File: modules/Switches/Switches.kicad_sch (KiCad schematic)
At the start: 0 parts

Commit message: Switches - module design - wip
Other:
- title: Eurorack [thing] -> Switches
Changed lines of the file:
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@@
   (paper "A4")
   (title_block
-    (title "Eurorack [thing]")
-    (rev "0.1")
+    (title "Switches")
+    (date "2023-10-12")
+    (rev "1.0")
     (company "Len Popp")
     (comment 1 "Copyright © 2023 Len Popp CC BY")
-    (comment 2 "Eurorack [thing] module - 8HP")
+    (comment 2 "Eurorack muting module module - 8HP")
   )
   (text "All fixed resistors are 1% tolerance unless otherwise specified.\nAll eletrolytic capacitors are rated for 25VDC unless otherwise specified."

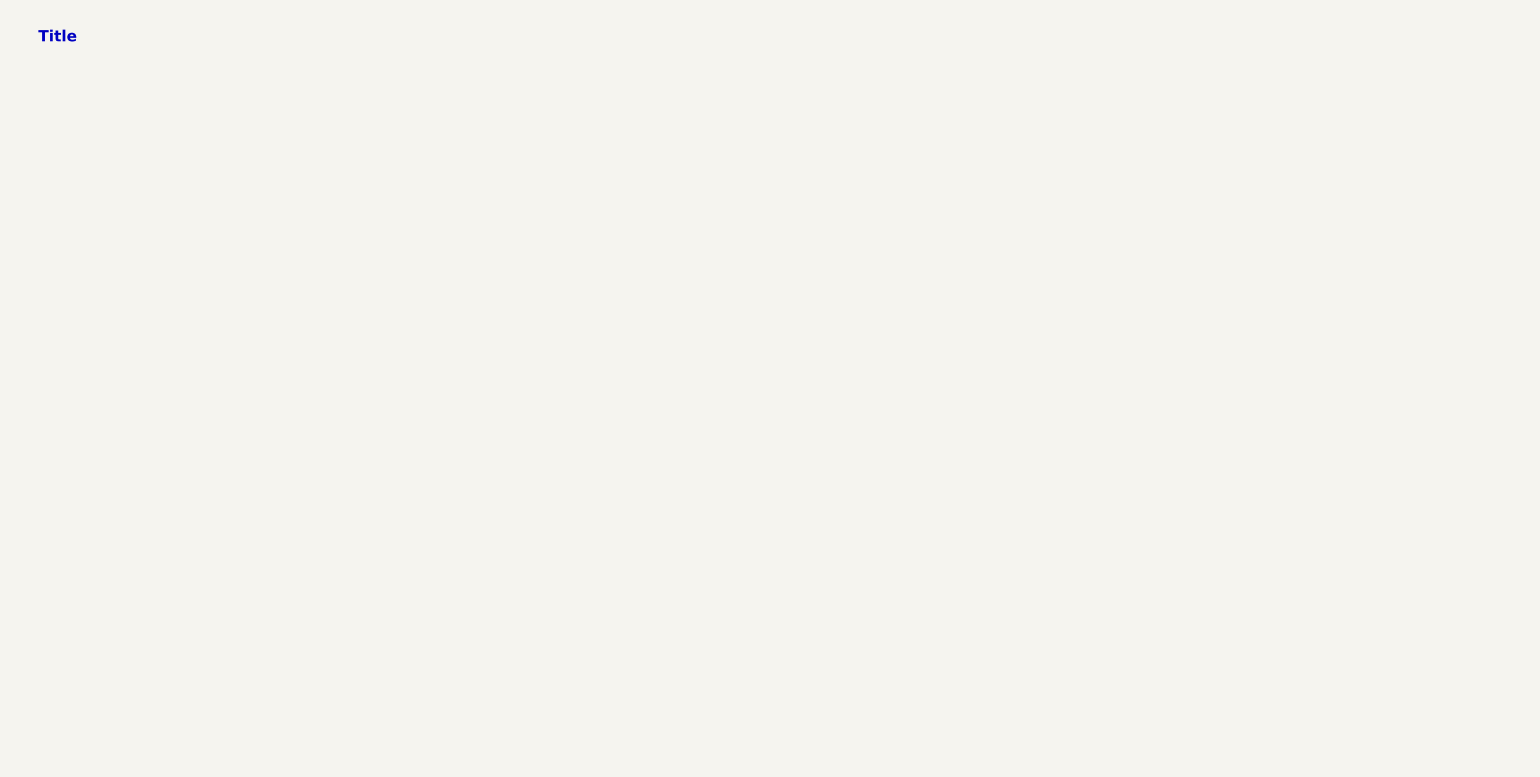
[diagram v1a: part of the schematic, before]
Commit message: Switches - module design - wip
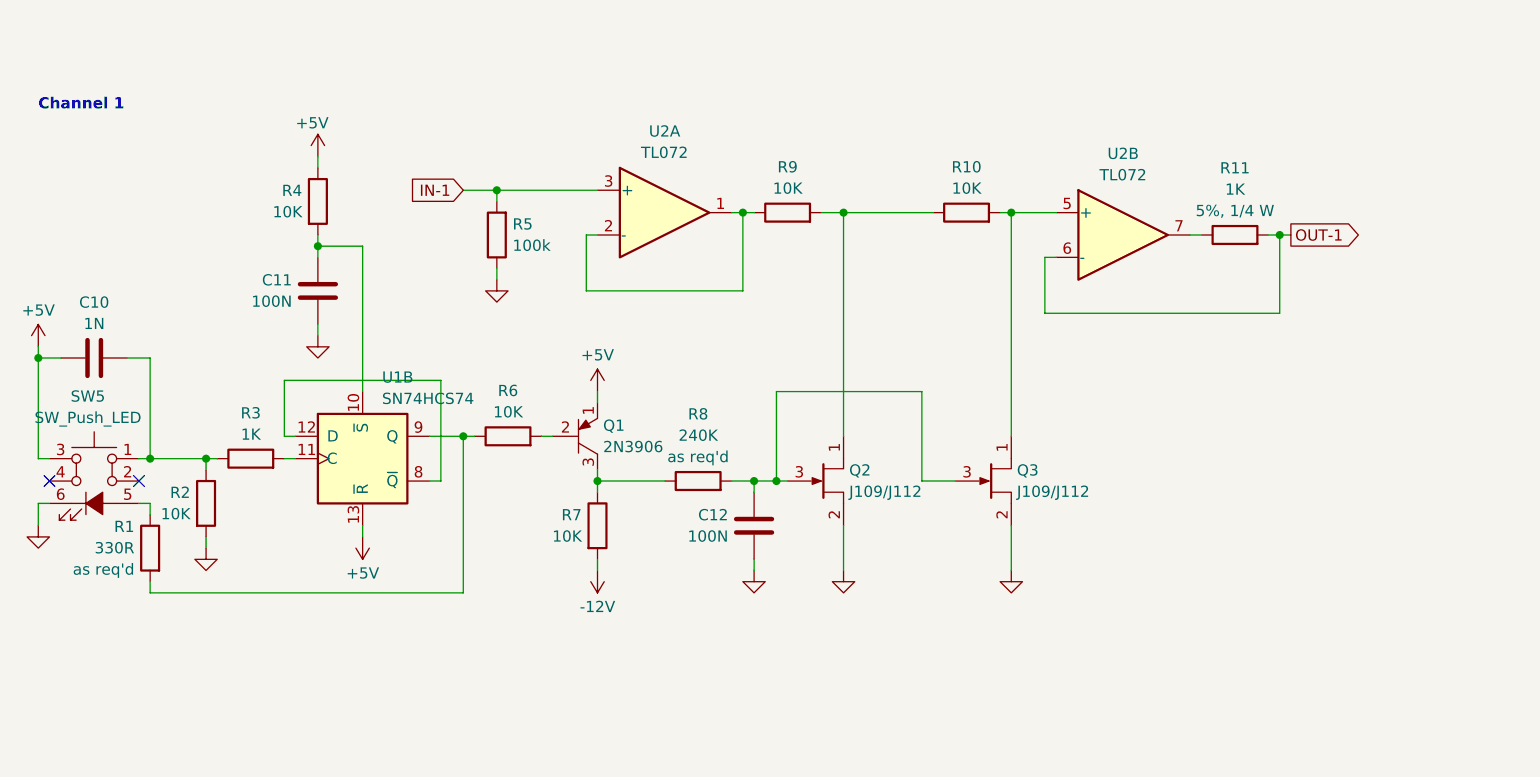
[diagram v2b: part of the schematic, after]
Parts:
- added C10: 1N, -lmp-stripboard:SB_Gen_2, symbol -lmp:CC_100N
- added C11, C12: 100N, -lmp-misc:C_Disc_D5.0mm_W2.5mm_P2.50mm, symbol -lmp:CC_100N
- added Q1: 2N3906, -lmp-misc:TO-92_Inline_Wide, symbol -lmp:Q_PNP_2N3906
- added Q2, Q3: J109/J112, -lmp-misc:TO-92_Inline_Wide, symbol -lmp:Q_JFET_N_DSG
- added R1: 330R, -lmp-stripboard:SB_Gen_1, symbol -lmp-synth:R_1K_Output
- added R10, R4, R9: 10K, -lmp-misc:R_Axial_DIN0207_L6.3mm_D2.5mm_P7.62mm_Horizontal, symbol -lmp:R_1%_0W166
- added R11: 1K, -lmp-stripboard:SB_Gen_2, symbol -lmp-synth:R_1K_Output
- added R2: 10K, -lmp-stripboard:SB_Gen_1, symbol -lmp:R_1%_0W166
- added R3: 1K, -lmp-stripboard:SB_Gen_1, symbol -lmp:R_1%_0W166
- added R5: 100k, -lmp-stripboard:SB_Gen_1, symbol -lmp:R_1%_0W166
- added R6, R7: 10K, -lmp-stripboard:SB_Gen_2, symbol -lmp:R_1%_0W166
- added R8: 240K, -lmp-stripboard:SB_Gen_2, symbol -lmp:R_1%_0W166
- added SW5: SW_Push_LED, -lmp-synth:SW_Push_LED_C&K_D6R, symbol -lmp-synth:SW_Push_LED_C&K_D6R
- added U1: SN74HCS74, -lmp-breakout:Breakout_DIP-14_W15.24mm, symbol -lmp-IC-misc:SN74HCS74
- added U2: TL072, Package_DIP:DIP-8_W7.62mm, symbol -lmp-opamp:TL072
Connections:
- new net: C10.2, R2.1, R3.1, SW5.1
- new net: R1.1, SW5.5 (A)
- new net: Q3.1 (D), R10.2, U2.5 (+)
- new net: C12.1, Q2.3 (G), Q3.3 (G), R8.2
- new net: R9.1, U2.1, U2.2 (-)
- new net: Q2.1 (D), R10.1, R9.2
- new net: R1.2, R6.1, U1.9 (Q)
- new net: Q1.2 (B), R6.2
- new net: Q1.3 (C), R7.1, R8.1
- new net: C11.1, R4.2, U1.10 (~{S})
- new net: R11.1, U2.7
- new net: R3.2, U1.11 (C)
- new net: U1.12 (D), U1.8 (~{Q})
- new net +5V: C10.1, Q1.1 (E), R4.1, SW5.3, U1.13 (~{R})
- new net -12V: R7.2
- new net GND: C11.2, C12.2, Q2.2 (S), Q3.2 (S), R2.2, R5.1, SW5.6 (K)
- new net IN-1: R5.2, U2.3 (+)
- new net OUT-1: R11.2, U2.6 (-)
- no-connect marks 0 -> 2
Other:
- note added: "Channel 1"
- note removed: "Title"

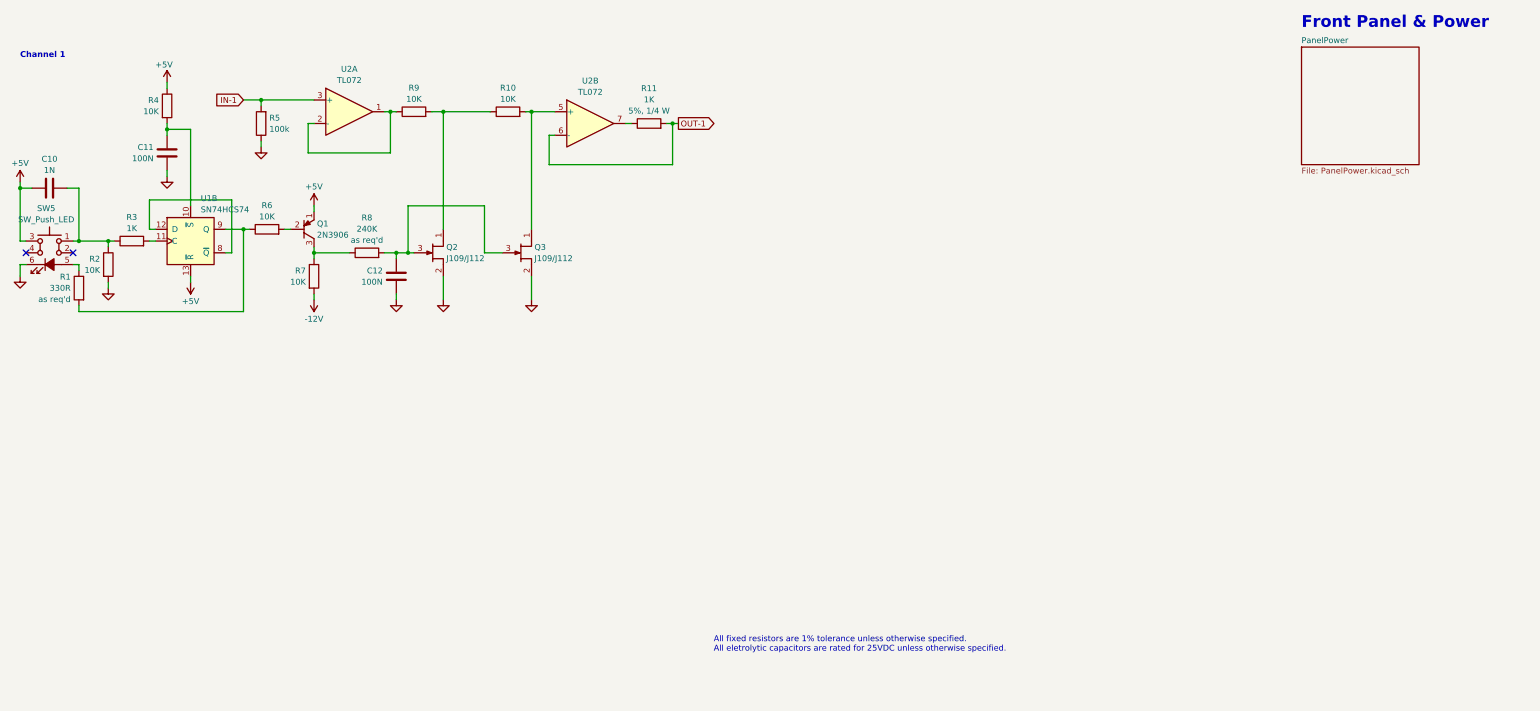
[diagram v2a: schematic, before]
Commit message: Switches - module design - wip
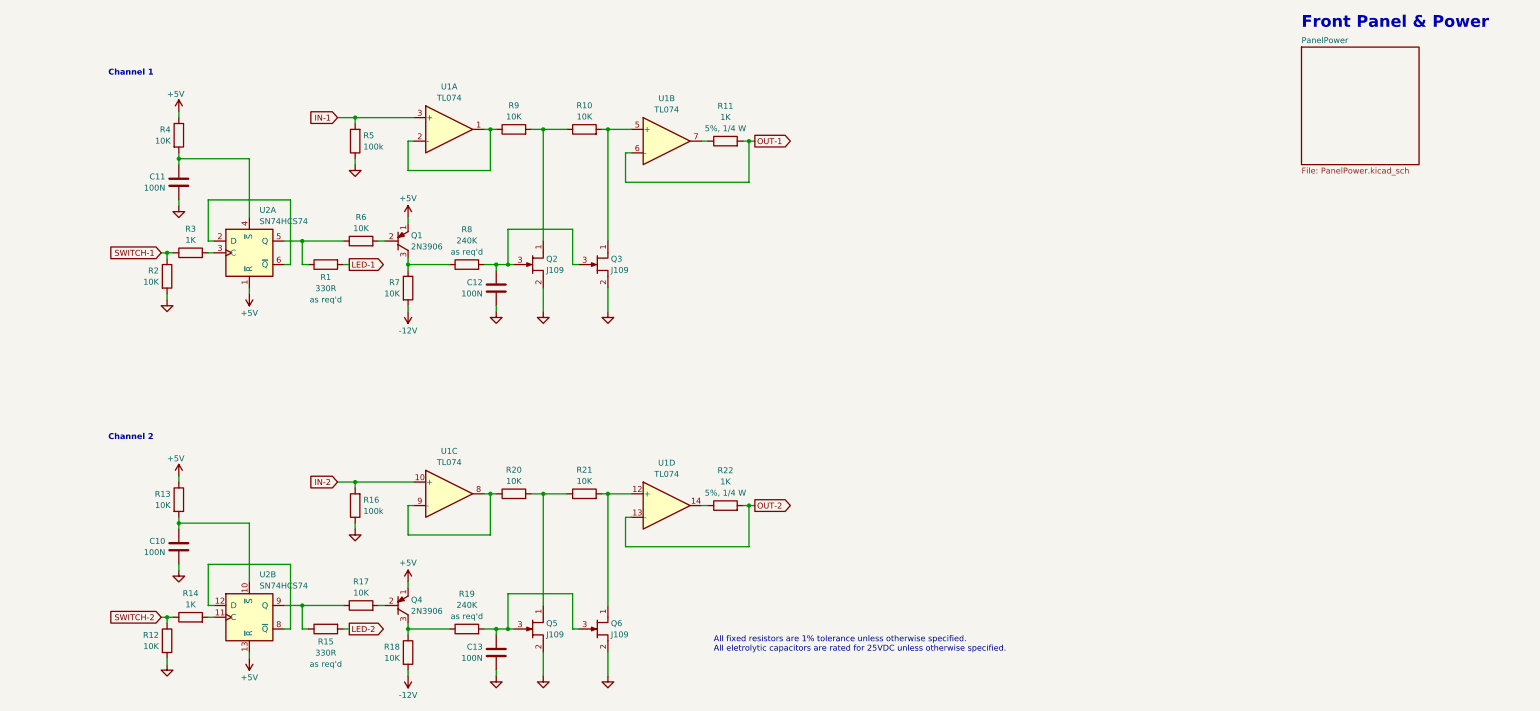
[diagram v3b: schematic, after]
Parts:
- removed SW5: SW_Push_LED, -lmp-synth:SW_Push_LED_C&K_D6R, symbol -lmp-synth:SW_Push_LED_C&K_D6R
- removed U2: TL072, Package_DIP:DIP-8_W7.62mm, symbol -lmp-opamp:TL072
- added C13: 100N, -lmp-misc:C_Disc_D5.0mm_W2.5mm_P2.50mm, symbol -lmp:CC_100N
- added Q4: 2N3906, -lmp-misc:TO-92_Inline_Wide, symbol -lmp:Q_PNP_2N3906
- added Q5, Q6: J109, -lmp-misc:TO-92_Inline_Wide, symbol -lmp:Q_JFET_N_DSG
- added R12: 10K, -lmp-stripboard:SB_Gen_1, symbol -lmp:R_1%_0W166
- added R13, R20, R21: 10K, -lmp-misc:R_Axial_DIN0207_L6.3mm_D2.5mm_P7.62mm_Horizontal, symbol -lmp:R_1%_0W166
- added R14: 1K, -lmp-stripboard:SB_Gen_1, symbol -lmp:R_1%_0W166
- added R15: 330R, -lmp-stripboard:SB_Gen_1, symbol -lmp-synth:R_1K_Output
- added R16: 100k, -lmp-stripboard:SB_Gen_1, symbol -lmp:R_1%_0W166
- added R17, R18: 10K, -lmp-stripboard:SB_Gen_2, symbol -lmp:R_1%_0W166
- added R19: 240K, -lmp-stripboard:SB_Gen_2, symbol -lmp:R_1%_0W166
- added R22: 1K, -lmp-stripboard:SB_Gen_2, symbol -lmp-synth:R_1K_Output
- added U1: TL074, Package_DIP:DIP-14_W7.62mm, symbol -lmp-opamp:TL074
- added unit 2 of U2
- C10: value 1N -> 100N; footprint -lmp-stripboard:SB_Gen_2 -> -lmp-misc:C_Disc_D5.0mm_W2.5mm_P2.50mm
- Q2, Q3: value J109/J112 -> J109
- renumbered U1 to U2
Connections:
- net +5V: now also U2.1 (~{R}), Q4.1 (E), R13.1, U2.13 (~{R}); no longer C10.1, U2.13 (~{R})
- net -12V: now also R18.2
- net GND: now also C10.2, C13.2, Q5.2 (S), Q6.2 (S), R12.2, R16.1
- net IN-1: now also U1.3 (+)
- net OUT-1: now also U1.6 (-)
- net SWITCH-1: now reaches R2.1, R3.1
- net SWITCH-1: no longer C10.2
- net at R1.1: now also R6.1, U2.5 (Q)
- net at Q3.1 (D), R10.2: now also U1.5 (+)
- net at R9.1: now also U1.1, U1.2 (-)
- net at C11.1, R4.2: now also U2.4 (~{S}); no longer U2.10 (~{S})
- net at R11.1: now also U1.7
- net at R3.2: now also U2.3 (C); no longer U2.11 (C)
- new net: R15.1, R17.1, U2.9 (Q)
- new net: Q4.2 (B), R17.2
- new net: R20.1, U1.8, U1.9 (-)
- new net: Q5.1 (D), R20.2, R21.1
- new net: Q4.3 (C), R18.1, R19.1
- new net: C10.1, R13.2, U2.10 (~{S})
- new net: R14.2, U2.11 (C)
- new net: U2.12 (D), U2.8 (~{Q})
- new net: Q6.1 (D), R21.2, U1.12 (+)
- new net: C13.1, Q5.3 (G), Q6.3 (G), R19.2
- new net: R22.1, U1.14
- new net: U2.2 (D), U2.6 (~{Q})
- new net IN-2: R16.2, U1.10 (+)
- new net LED-1: R1.2
- new net LED-2: R15.2
- new net OUT-2: R22.2, U1.13 (-)
- new net SWITCH-2: R12.1, R14.1
- no-connect marks 2 -> 0
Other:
- note added: "Channel 2"
- moved on the sheet: C11, C12, Q1, Q2, Q3, R1, R10, R11, R2, R3, R4, R5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
